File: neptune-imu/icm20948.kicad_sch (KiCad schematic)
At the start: 4 parts, among them U2 ICM-20948

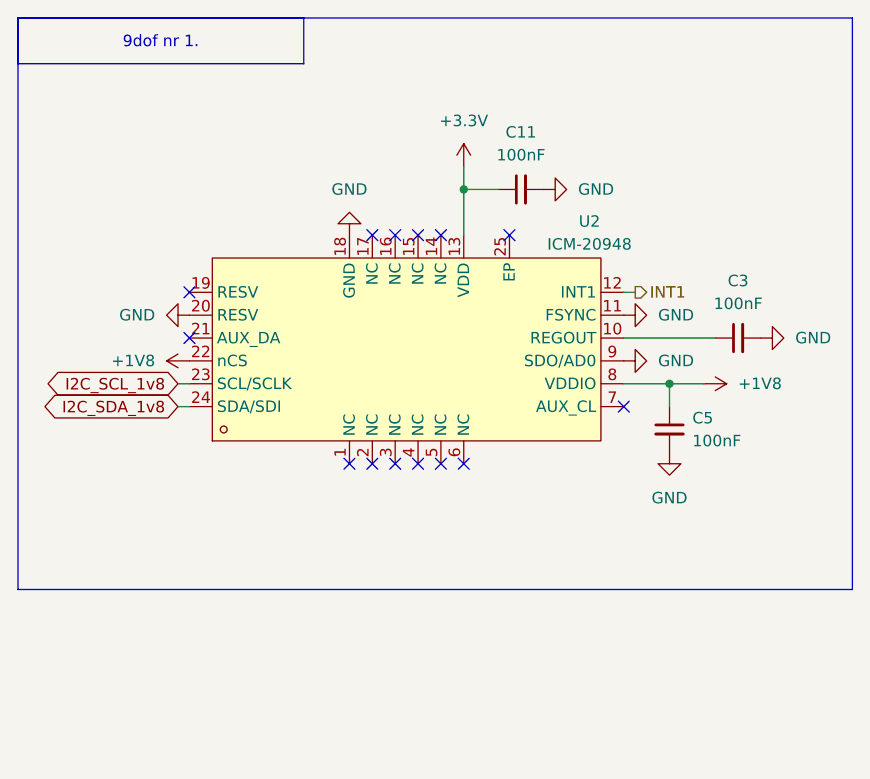
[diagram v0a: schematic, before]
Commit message: going to school
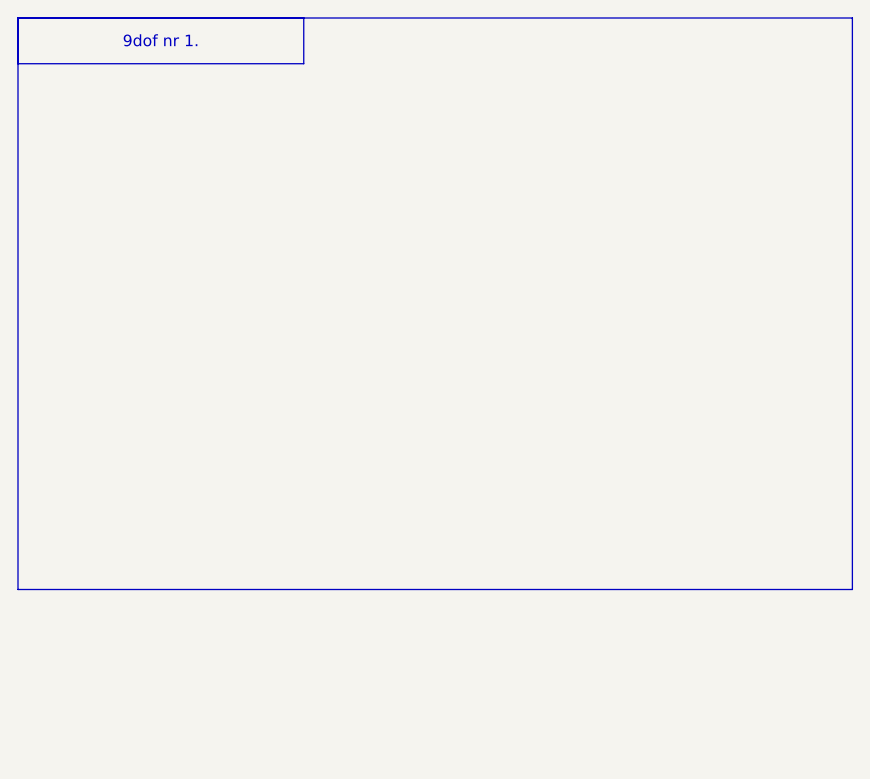
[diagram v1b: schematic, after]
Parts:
- removed C11, C3, C5: 100nF, symbol Device:C_Small
- removed U2: ICM-20948, cigo:QFN-24_L3.0-W3.0-P0.40-BL-EP, symbol neptune-imu-symbols:ICM-20948
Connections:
- no-connect marks 14 -> 0

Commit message: final
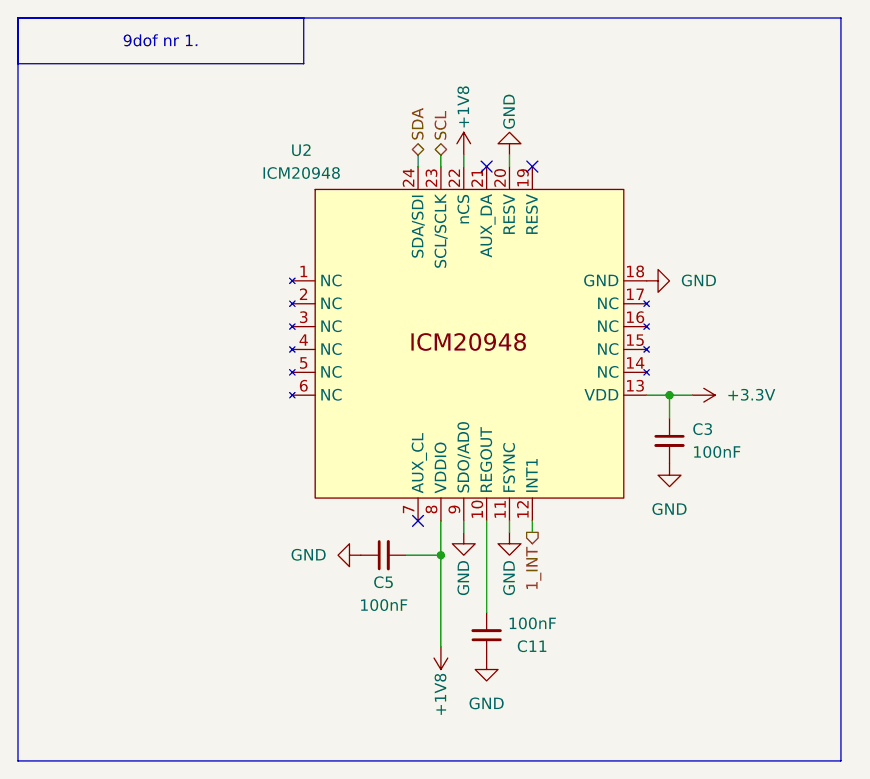
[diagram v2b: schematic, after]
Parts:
- added C11, C3, C5: 100nF, Capacitor_SMD:C_0402_1005Metric, symbol Device:C_Small
- added U2: ICM20948, neptune-imu-footprints:icm20948, symbol neptune-imu-symbols:ICM20948
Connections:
- new net: C11.2, U2.10 (REGOUT)
- new net +1V8: C5.2, U2.22 (nCS), U2.8 (VDDIO)
- new net +3.3V: C3.1, U2.13 (VDD)
- new net 1_INT: U2.12 (INT1)
- new net GND: C11.1, C3.2, C5.1, U2.11 (FSYNC), U2.18 (GND), U2.20 (RESV), U2.9 (SDO/AD0)
- new net SCL: U2.23 (SCL/SCLK)
- new net SDA: U2.24 (SDA/SDI)
- no-connect marks 0 -> 3
